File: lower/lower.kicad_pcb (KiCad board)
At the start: 2 copper layers, 187 x 130 mm, 36 parts, among them M1 MotorCutout, M2 MotorCutout, M3 MotorCutout, M4 MotorCutout, SW1 SW_SPDT, U1 BTS50080-1TMA

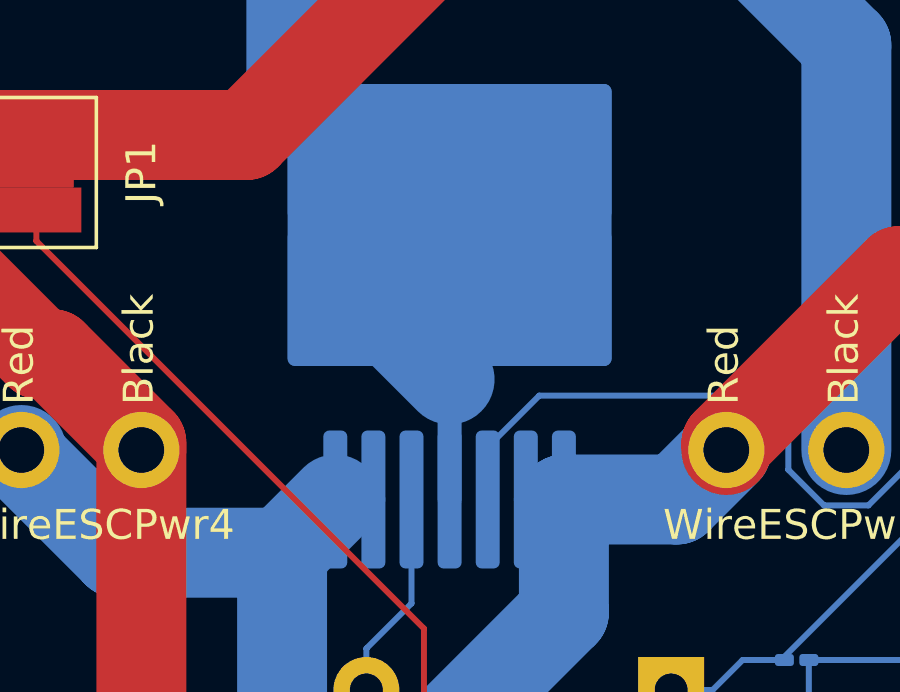
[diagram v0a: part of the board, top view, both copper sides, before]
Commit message: Lower: v0.2.1. Routed
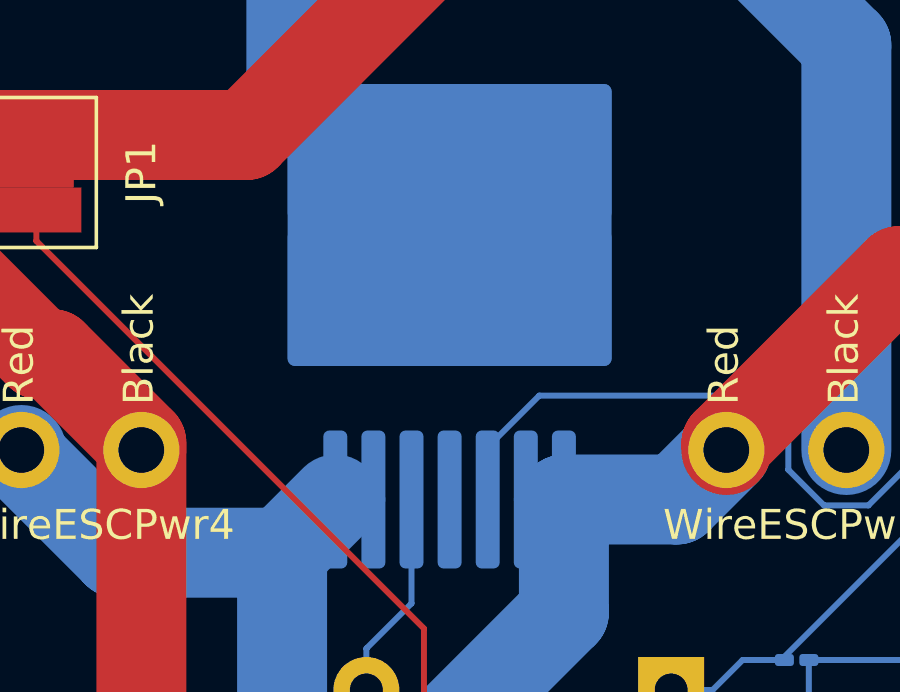
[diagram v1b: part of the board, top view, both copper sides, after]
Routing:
- net /Vbb: track 35.4 -> 24.1 mm
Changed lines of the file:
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@@
 			(drillshape 0)
 			(scaleselection 1)
-			(outputdirectory "C:/Users/engi/Documents/kicad_projects/nano_quadcopter/lower/lower_v0.1.0/")
+			(outputdirectory "C:/Users/engi/Documents/kicad_projects/nano_quadcopter/lower/v0.2.0/")
 		)
 	)
@@
 	)
 	(segment
-		(start 167.125 42.5)
-		(end 169.55 44.925)
-		(width 3)
-		(layer "B.Cu")
-		(net 7)
-	)
-	(segment
-		(start 164.0264 44.8986)
-		(end 166.775 47.6473)
-		(width 3)
-		(layer "B.Cu")
-		(net 7)
-	)
-	(segment
 		(start 164 40.075)
 		(end 166.425 42.5)
@@
 		(layer "B.Cu")
 		(net 7)
-	)
-	(segment
-		(start 166.775 47.6473)
-		(end 166.775 51.65)
-		(width 0.8014)
-		(layer "B.Cu")
-		(net 7)
